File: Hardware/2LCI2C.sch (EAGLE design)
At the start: 37 parts, among them IC1 NAU7802-SOIC, IC2 HX711-SOP16L, IC3 TCA9548A, J3 Load Cell, J4 Load Cell, Q2 2N3906

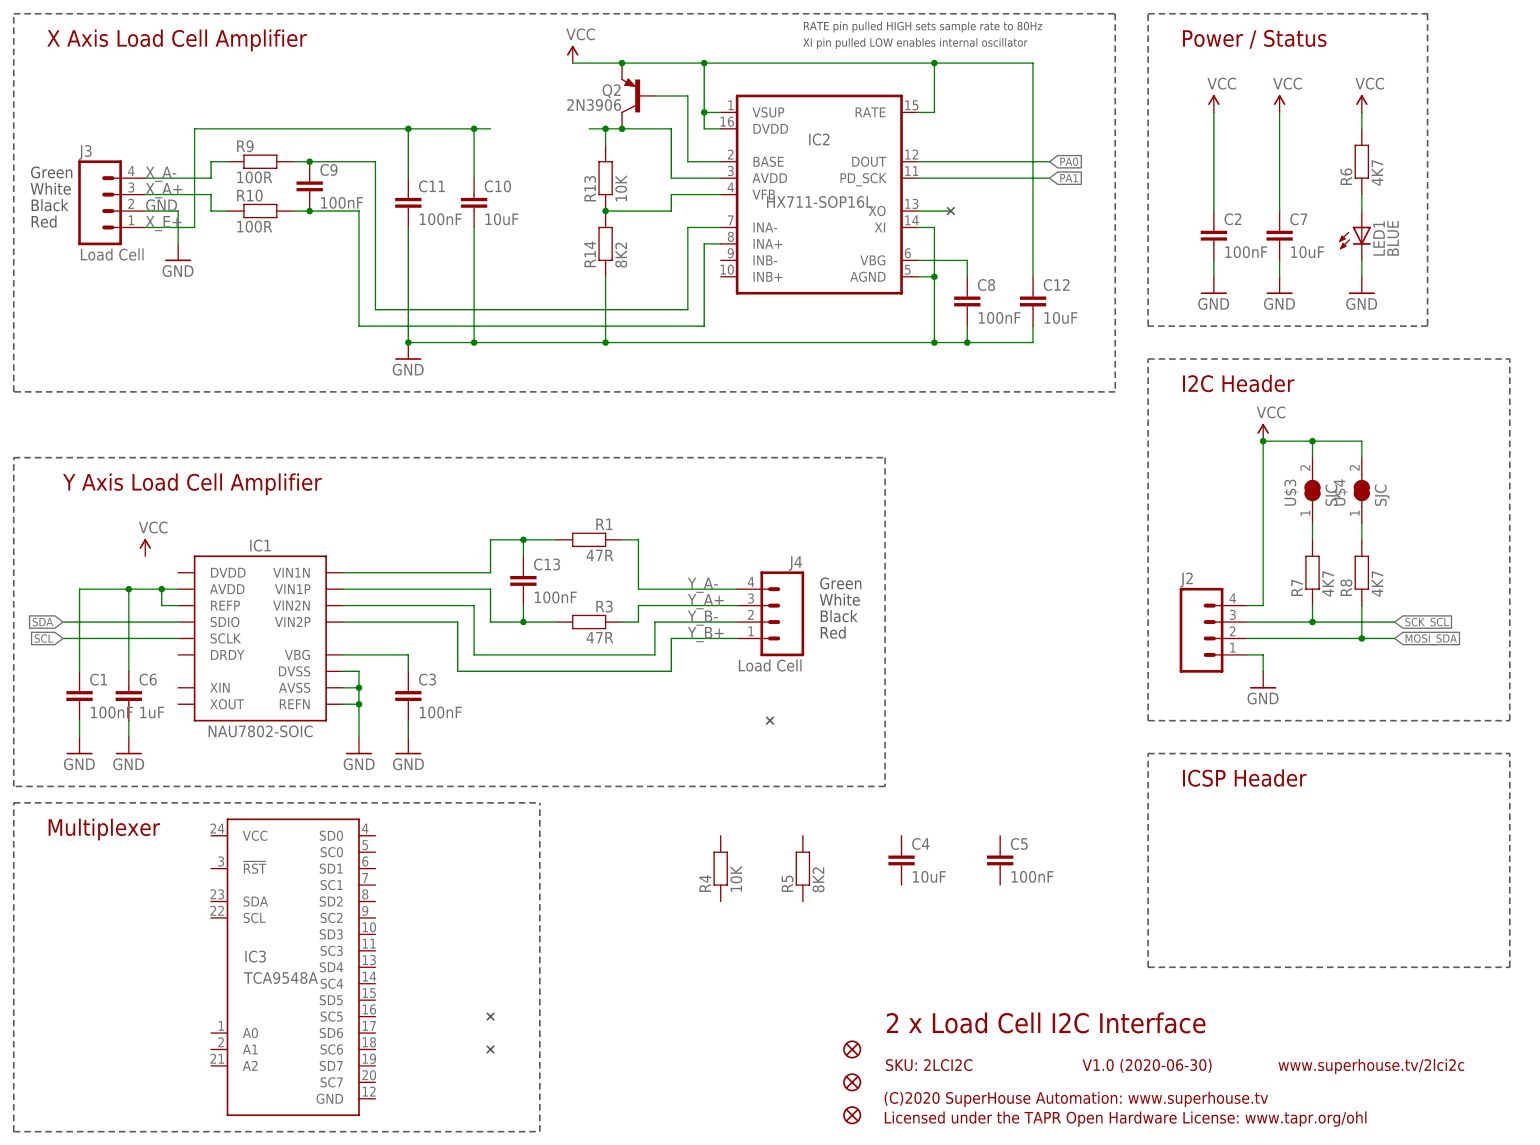
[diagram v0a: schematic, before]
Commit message: Partial conversion of early concept PCB.
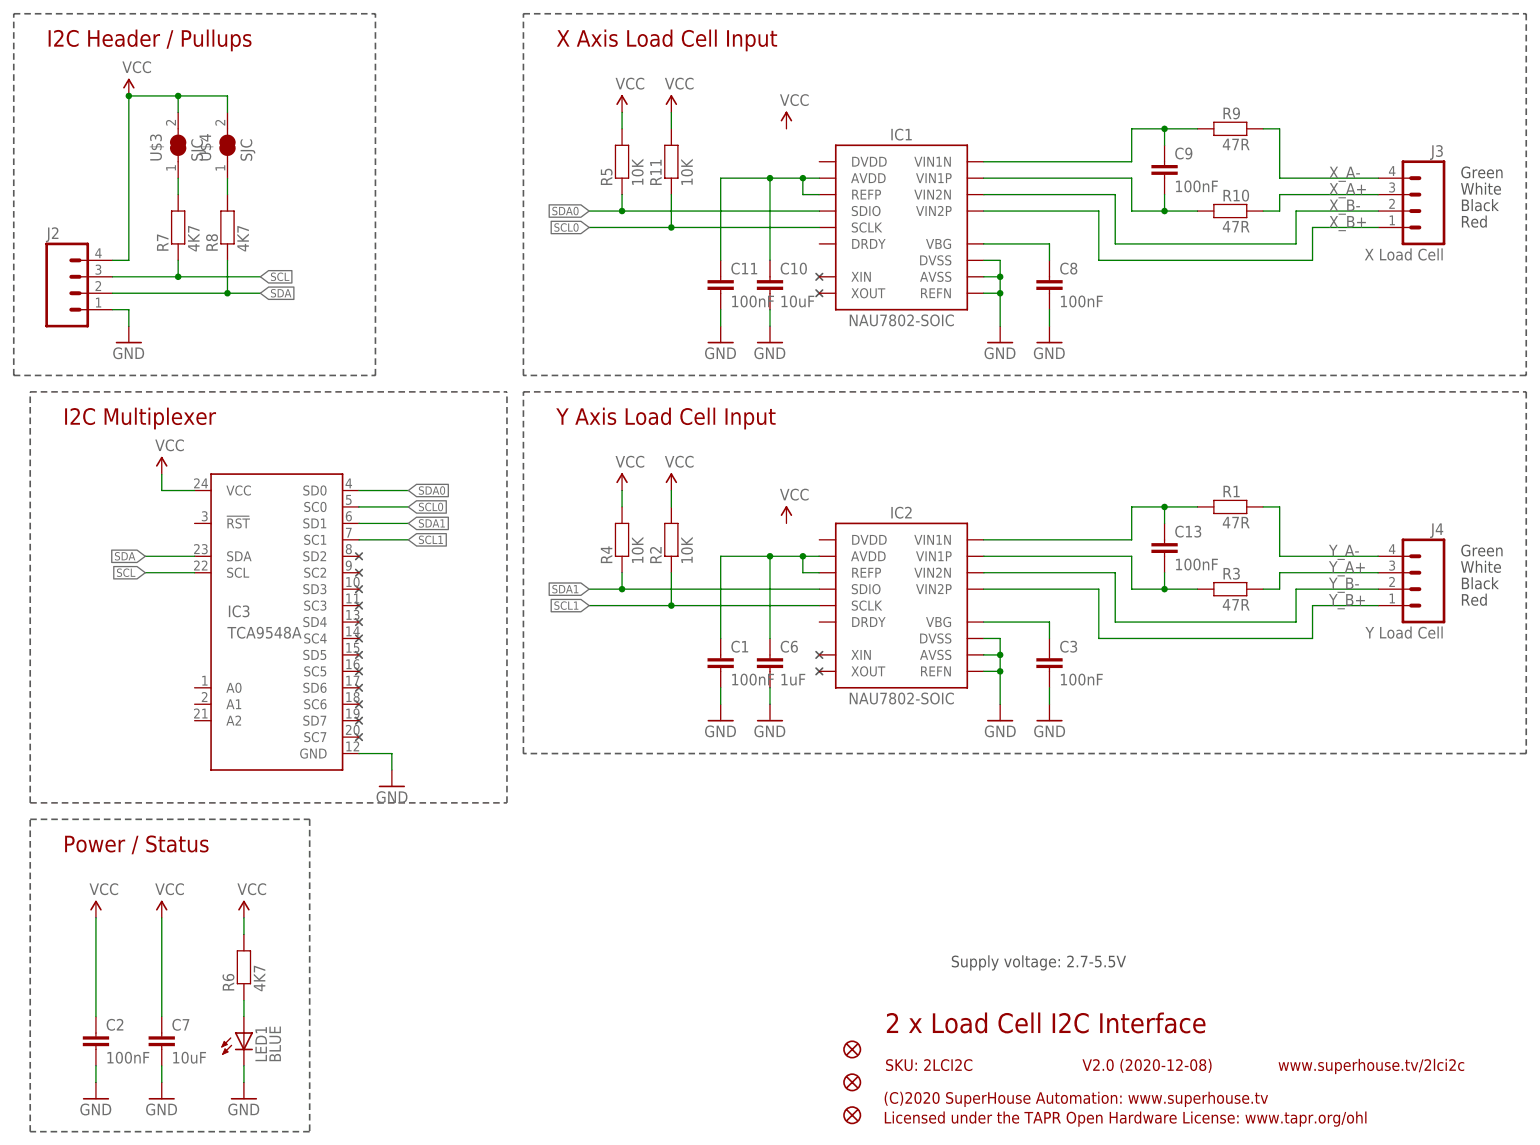
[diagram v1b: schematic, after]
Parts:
- removed C12, C4: 10uF, SuperHouse-DiscreteSemi:CAP0805
- removed C5: 100nF, SuperHouse-DiscreteSemi:CAP0603
- removed Q2: 2N3906, SuperHouse-DiscreteSemi:TRANS_PNPMMBT3906LT1SOT23-BEC
- removed R13: 10K, SuperHouse-DiscreteSemi:RESISTOR0603
- removed R14: 8K2, SuperHouse-DiscreteSemi:RESISTOR0603
- added R11, R2: 10K, SuperHouse-DiscreteSemi:RESISTOR0603
- IC2: value HX711-SOP16L -> NAU7802-SOIC; device SuperHouse-ICs:HX711-SOP16L -> SuperHouse-ICs:NAU7802-SOIC
- J3: value Load Cell -> X Load Cell
- J4: value Load Cell -> Y Load Cell
- R10, R9: value 100R -> 47R
- R5: value 8K2 -> 10K
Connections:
- removed net MOSI_SDA: J2.2, R8.1
- removed net N$14: C9.1, IC2.INA-, R9.2
- removed net N$15: C9.2, IC2.INA+, R10.2
- removed net N$16: IC2.AVDD, Q2.C, R13.2
- removed net N$17: C8.1, IC2.VBG
- removed net N$20: IC2.BASE, Q2.B
- removed net N$21: IC2.VFB, R13.1, R14.2
- removed net PA0: IC2.DOUT
- removed net PA1: IC2.PD_SCK
- removed net SCK_SCL: J2.3, R7.1
- removed net X_E+: C10.1, C11.1, J3.1
- new net N$6: C9.1, IC1.VIN1N, R9.1
- new net N$7: C9.2, IC1.VIN1P, R10.1
- new net N$9: C10.1, C11.1, IC1.AVDD, IC1.REFP
- new net SCL0: IC1.SCLK, IC3.SC0, R11.1
- new net SCL1: IC2.SCLK, IC3.SC1, R2.1
- new net SDA0: IC1.SDIO, IC3.SD0, R5.1
- new net SDA1: IC2.SDIO, IC3.SD1, R4.1
- new net X_B+: IC1.VIN2P, J3.1
- new net X_B-: IC1.VIN2N, J3.2
- net GND: now also IC2.AVSS, IC2.DVSS, IC2.REFN, IC3.GND; no longer C12.2, IC2.AGND, IC2.XI, J3.2, R14.1
- net N$1: now also IC2.VBG; no longer IC1.VBG
- net N$2: now also IC2.VIN1N, R1.1; no longer IC1.VIN1N, R1.2
- net N$3: now also IC2.AVDD, IC2.REFP; no longer IC1.AVDD, IC1.REFP
- net N$4: now also IC2.VIN1P, R3.1; no longer IC1.VIN1P, R3.2
- net N$8: now also C8.1, IC1.VBG; no longer IC2.XO
- net SCL: now also IC3.SCL, J2.3, R7.1; no longer IC1.SCLK
- net SDA: now also IC3.SDA, J2.2, R8.1; no longer IC1.SDIO
- net VCC: now also IC3.VCC, R11.2, R2.2, R4.2, R5.2; no longer C12.1, IC2.DVDD, IC2.RATE, IC2.VSUP, Q2.E
- net X_A+: now also R10.2; no longer R10.1
- net X_A-: now also R9.2; no longer R9.1
- net Y_A+: now also R3.2; no longer R3.1
- net Y_A-: now also R1.2; no longer R1.1
- net Y_B+: now also IC2.VIN2P; no longer IC1.VIN2P
- net Y_B-: now also IC2.VIN2N; no longer IC1.VIN2N
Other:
- note added: "I2C Header / Pullups"
- note added: "I2C Multiplexer"
- note added: "Supply voltage: 2.7-5.5V"
- note added: "V2.0 (2020-12-08)"
- note added: "X Axis Load Cell Input"
- note added: "Y Axis Load Cell Input"
- note removed: "I2C Header"
- note removed: "ICSP Header"
- note removed: "Multiplexer"
- note removed: "RATE pin pulled HIGH sets sample rate to 80Hz"
- note removed: "V1.0 (2020-06-30)"
- note removed: "X Axis Load Cell Amplifier"
- note removed: "XI pin pulled LOW enables internal oscillator"
- note removed: "Y Axis Load Cell Amplifier"
- moved on the sheet: C1, C10, C11, C13, C2, C3, C6, C7, C8, C9, IC1, IC3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
